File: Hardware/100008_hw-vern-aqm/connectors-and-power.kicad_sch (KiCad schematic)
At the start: 25 parts

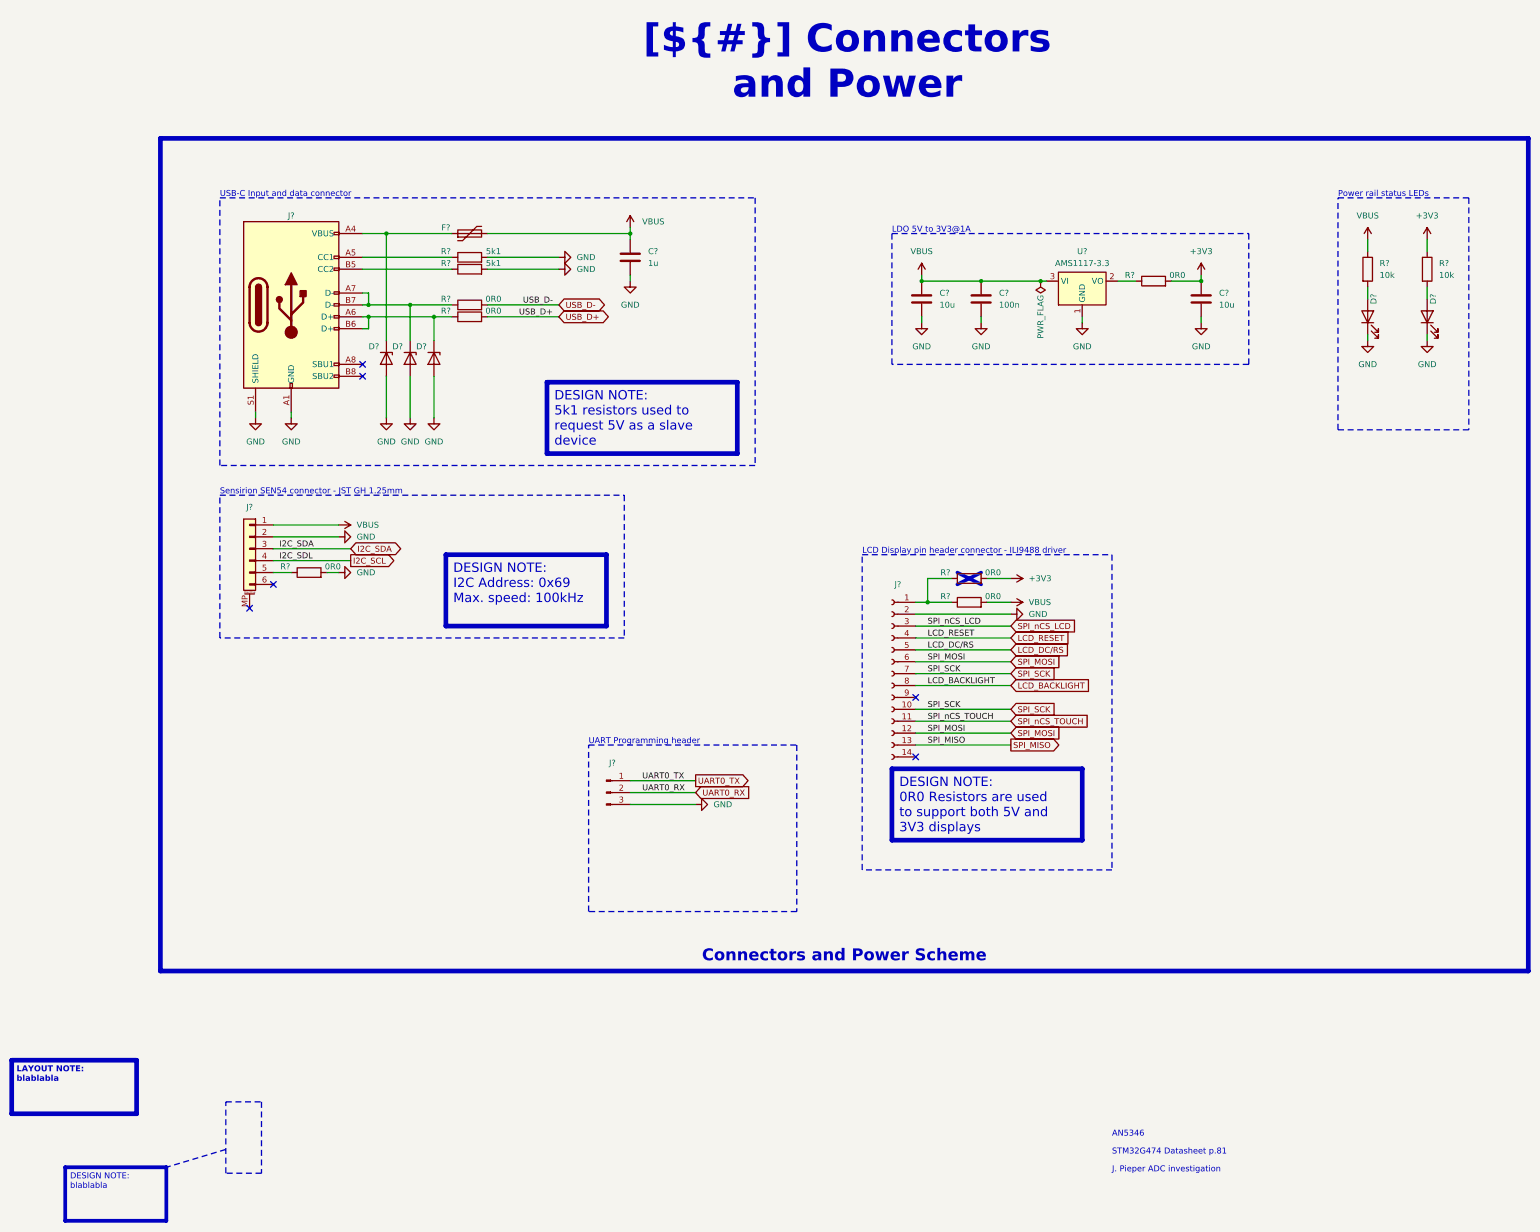
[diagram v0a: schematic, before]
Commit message: schematic work
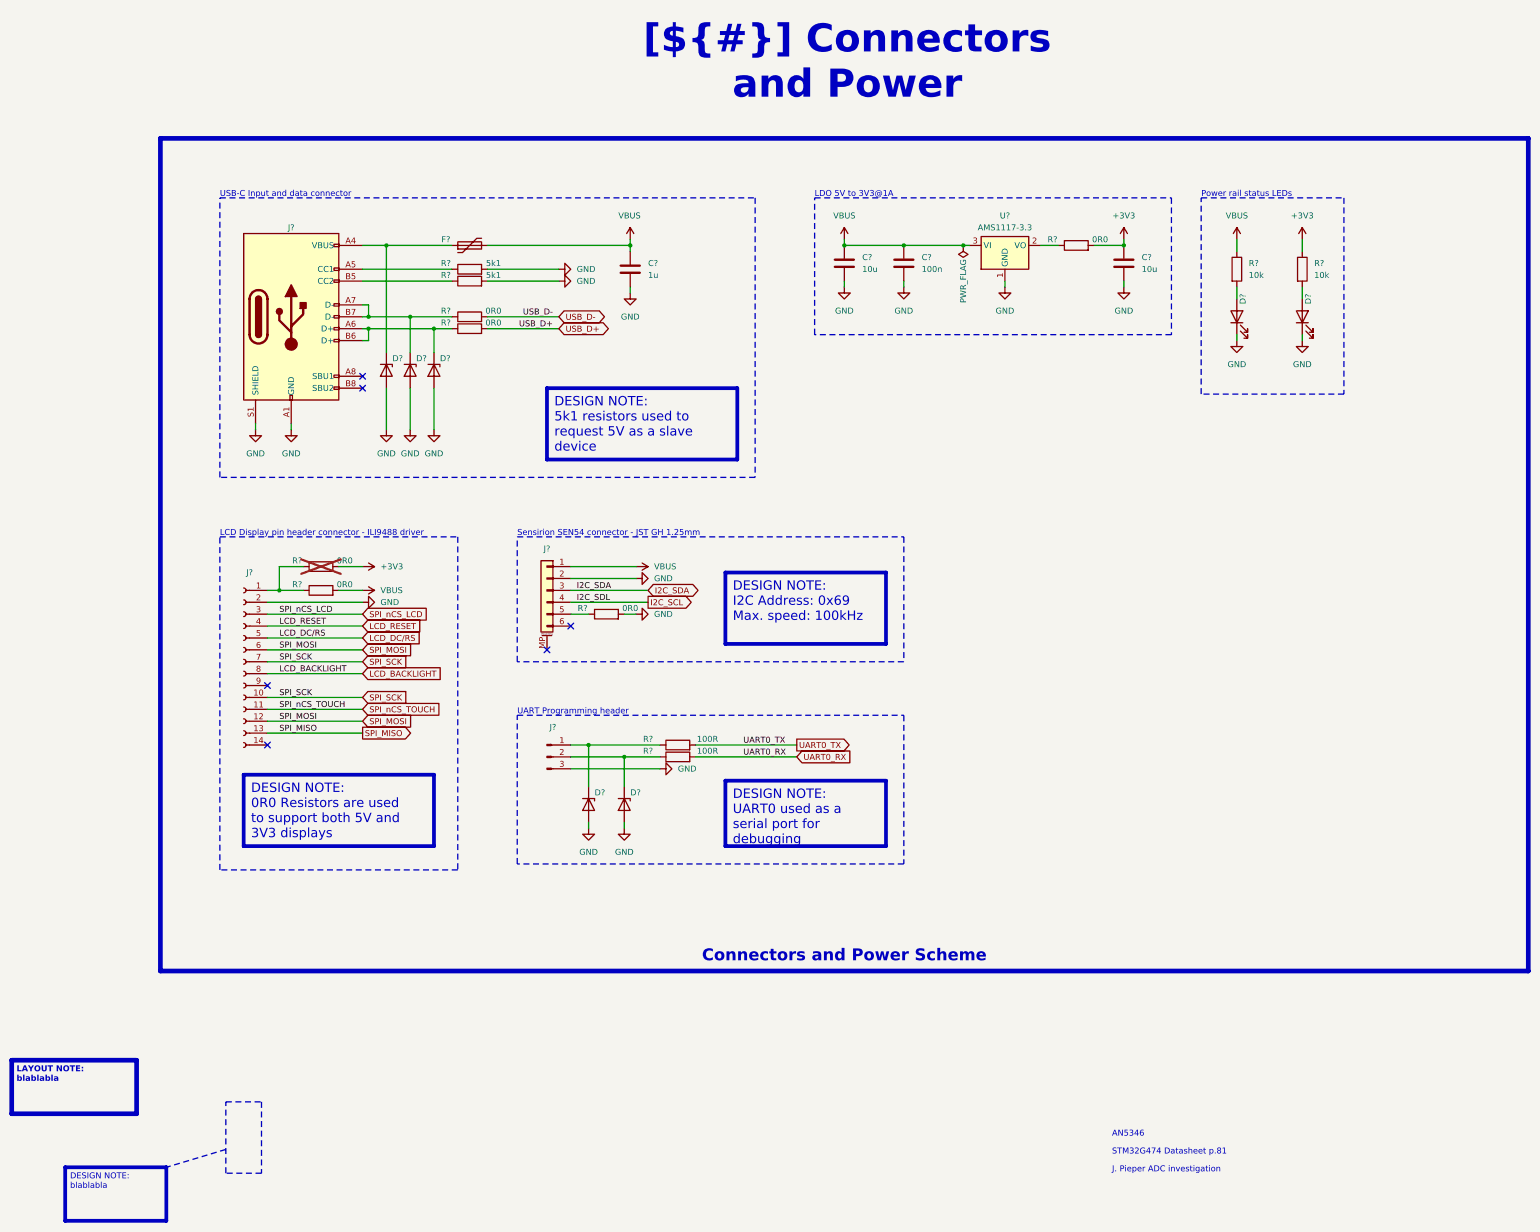
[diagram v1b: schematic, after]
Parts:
- removed D? (x2): ESD321, Diode_SMD:D_SOD-523, symbol Diode:ESD5Zxx
- added D? (x4): ESD321DYAR, Diode_SMD:D_SOD-523, symbol Active-Components:ESD321DYAR
- added R? (x2): 100R, Resistor_SMD:R_0603_1608Metric, symbol Device:R
- R?: now not fitted; now left out of the parts list
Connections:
- net GND: now also D?.2 (A), D?.2 (A), D?.2 (A), D?.2 (A)
- net UART0_RX: now also R?.2; no longer J?.2 (Pin_2)
- net UART0_TX: now also R?.2; no longer J?.1 (Pin_1)
- net at J?.A7 (D-), J?.B7 (D-), R?.1: now also D?.1 (K)
- net at J?.A6 (D+), J?.B6 (D+), R?.1: now also D?.1 (K)
- new net: D?.1 (K), J?.1 (Pin_1), R?.1
- new net: D?.1 (K), J?.2 (Pin_2), R?.1
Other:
- moved on the sheet: C?, D?, F?, J?, R?, U?

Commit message: schematic work
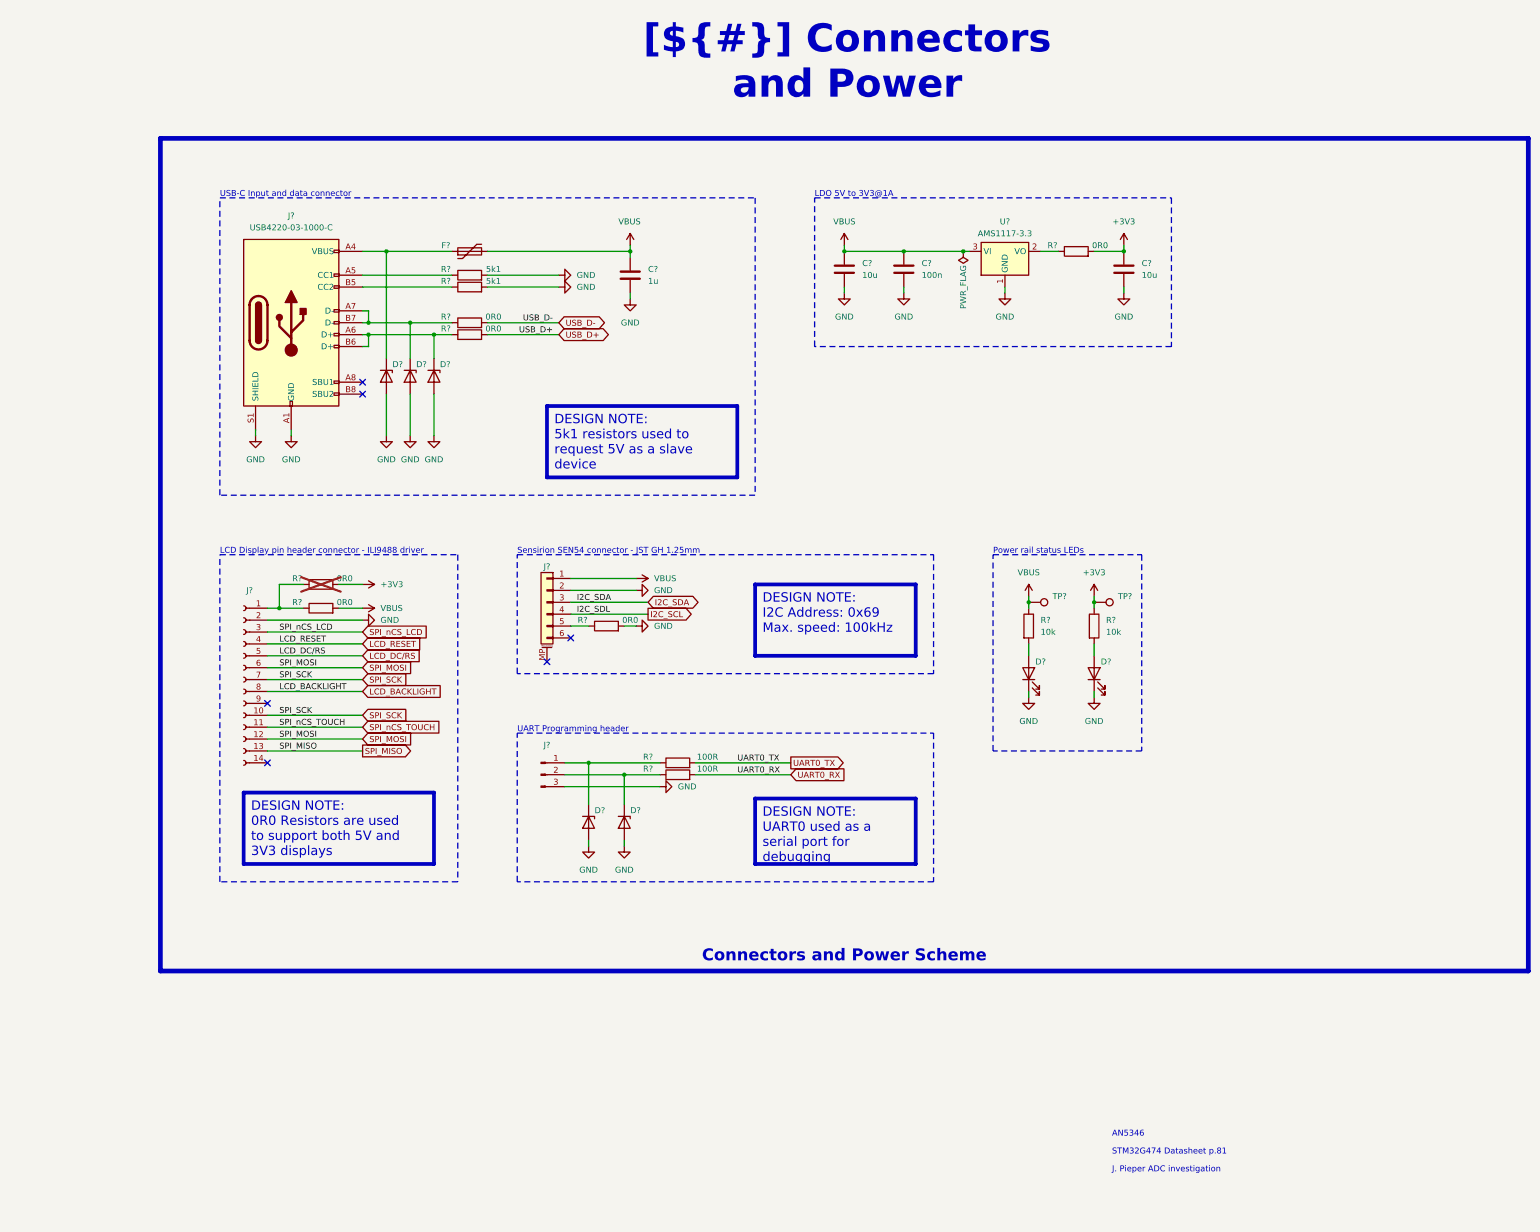
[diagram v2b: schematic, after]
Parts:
- removed D?: LED, LED_SMD:LED_0805_2012Metric, symbol Device:LED
- removed J?: USB_C_Receptacle_USB2.0_16P, symbol Connector:USB_C_Receptacle_USB2.0_16P
- added D?: LED, LED_SMD:LED_0603_1608Metric, symbol Device:LED
- added J?: USB4220-03-1000-C, Mechanical:USB_C_Receptacle_GCT_USB4220-03-xxxx-C_Vertical, symbol Mechanical-Parts:GCT_USB4220-03-1000-C
- added TP? (x2): TestPoint, TestPoint:TestPoint_Pad_D1.5mm, symbol Connector:TestPoint
- D?: footprint LED_SMD:LED_0805_2012Metric -> LED_SMD:LED_0603_1608Metric
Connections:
- net +3V3: now also TP?.1
- net GND: now also D?.1 (K), J?.A1 (GND), J?.A12 (GND), J?.B1 (GND), J?.B12 (GND), J?.S1 (SHIELD)
- net VBUS: now also TP?.1
- net at R?.2: now also D?.2 (A)
- net at R?.1: now also J?.B5 (CC2)
- net at D?.1 (K), R?.1: now also J?.A7 (D-), J?.B7 (D-)
- net at D?.1 (K), R?.1: now also J?.A6 (D+), J?.B6 (D+)
- net at D?.1 (K), F?.1: now also J?.A4 (VBUS), J?.A9 (VBUS), J?.B4 (VBUS), J?.B9 (VBUS)
- net at R?.1: now also J?.A5 (CC1)
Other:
- moved on the sheet: C?, D?, F?, J?, R?, U?
